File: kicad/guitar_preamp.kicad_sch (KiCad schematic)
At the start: 42 parts, among them J1 IN (от SW1B, экранир. провод), J2 BAT+ (TP4056 OUT+), J3 OUT (к SW1A) / GND, J4 Выход 6.3 стерео TRS, J5 Звукосниматели: COM/GND, J6 TP4056 OUT+/OUT-, J7 LED (A / K), SW1 DPDT push-pull RV1, U1 MCP6022/OPA2316

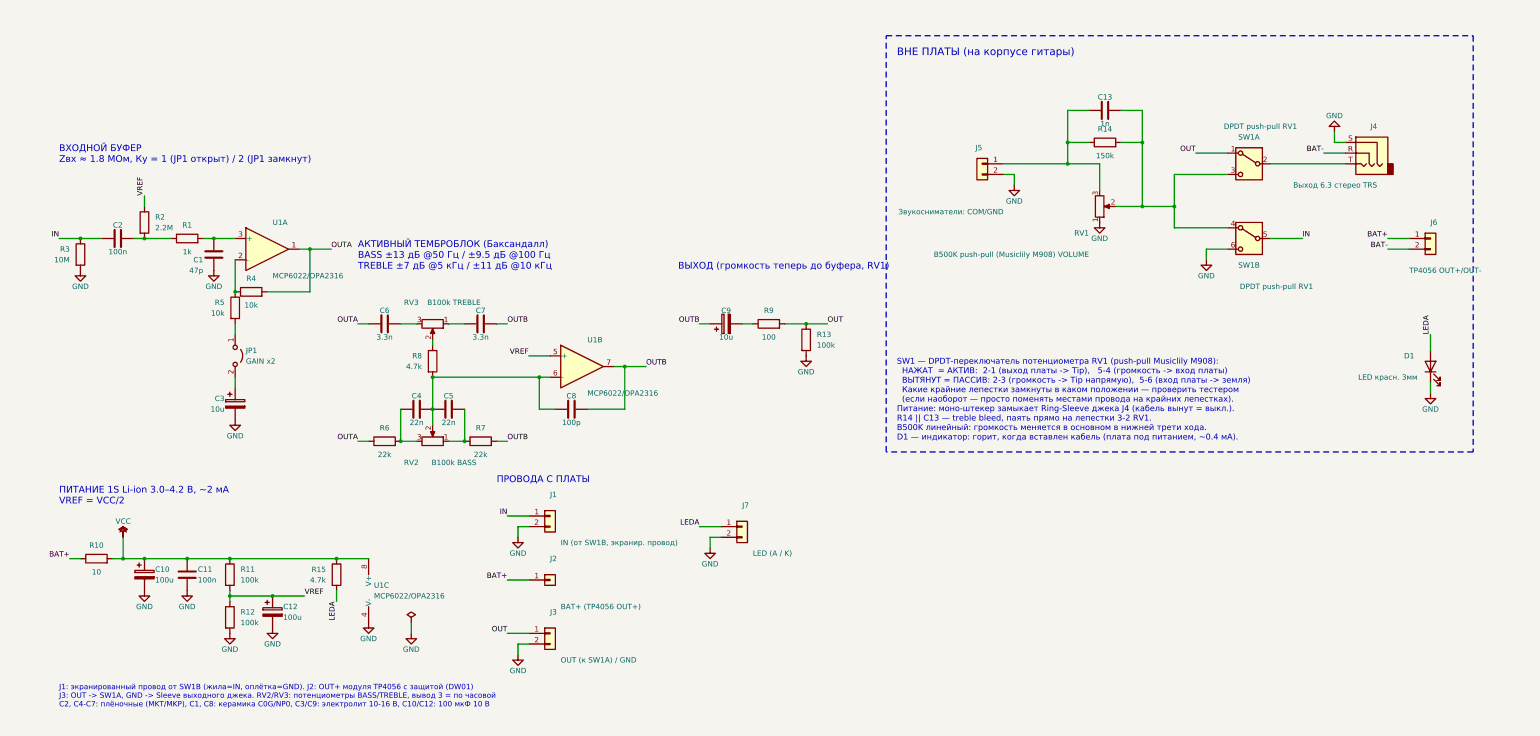
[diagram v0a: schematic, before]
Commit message: понятнее для меня подключение jeck
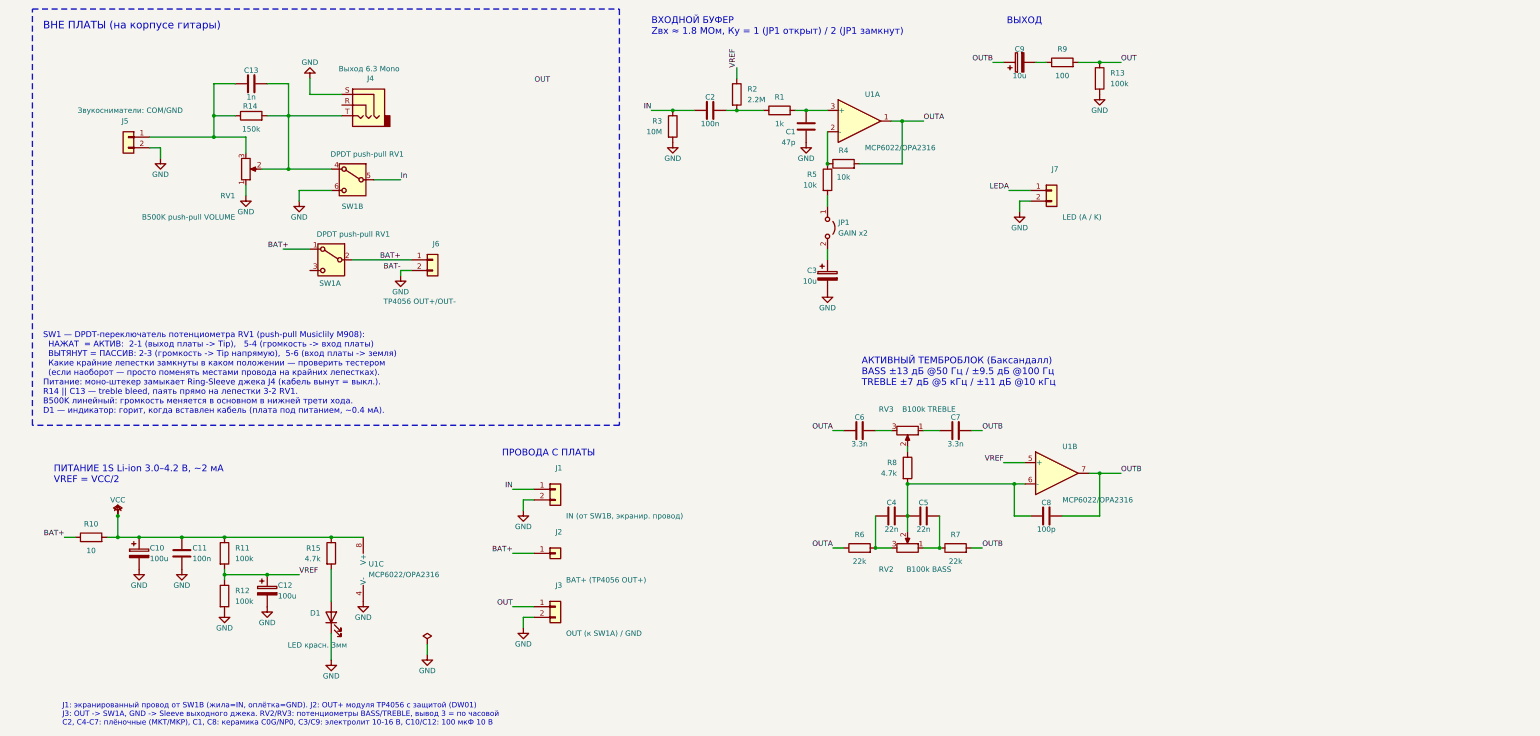
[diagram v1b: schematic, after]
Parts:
- J4: value Выход 6.3 стерео TRS -> Выход 6.3 Mono
- RV1: value B500K push-pull (Musiclily M908) VOLUME -> B500K push-pull VOLUME
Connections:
- net BAT+: now also SW1.1 (A), SW1.2 (B)
- net GND: now also J6.2 (Pin_2)
- net IN: no longer SW1.5 (B)
- net LEDA: no longer D1.2 (A), R15.2
- net OUT: no longer SW1.1 (A)
- net at C13.2, R14.2, RV1.2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: now also J4.T; no longer SW1.3 (C)
- net BAT-: no longer names the net of J4.R
- net BAT-: no longer J6.2 (Pin_2)
- new net: D1.2 (A), R15.2
- new net In: SW1.5 (B)
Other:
- note added: "ВЫХОД"
- note removed: "ВЫХОД (громкость теперь до буфера, RV1)"
- moved on the sheet: C1, C10, C11, C12, C13, C2, C3, C4, C5, C6, C7, C8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
